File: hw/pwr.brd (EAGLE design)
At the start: 30.6 x 25.4 mm, 20 parts, among them IC1 MAX640, IC2 MAX640

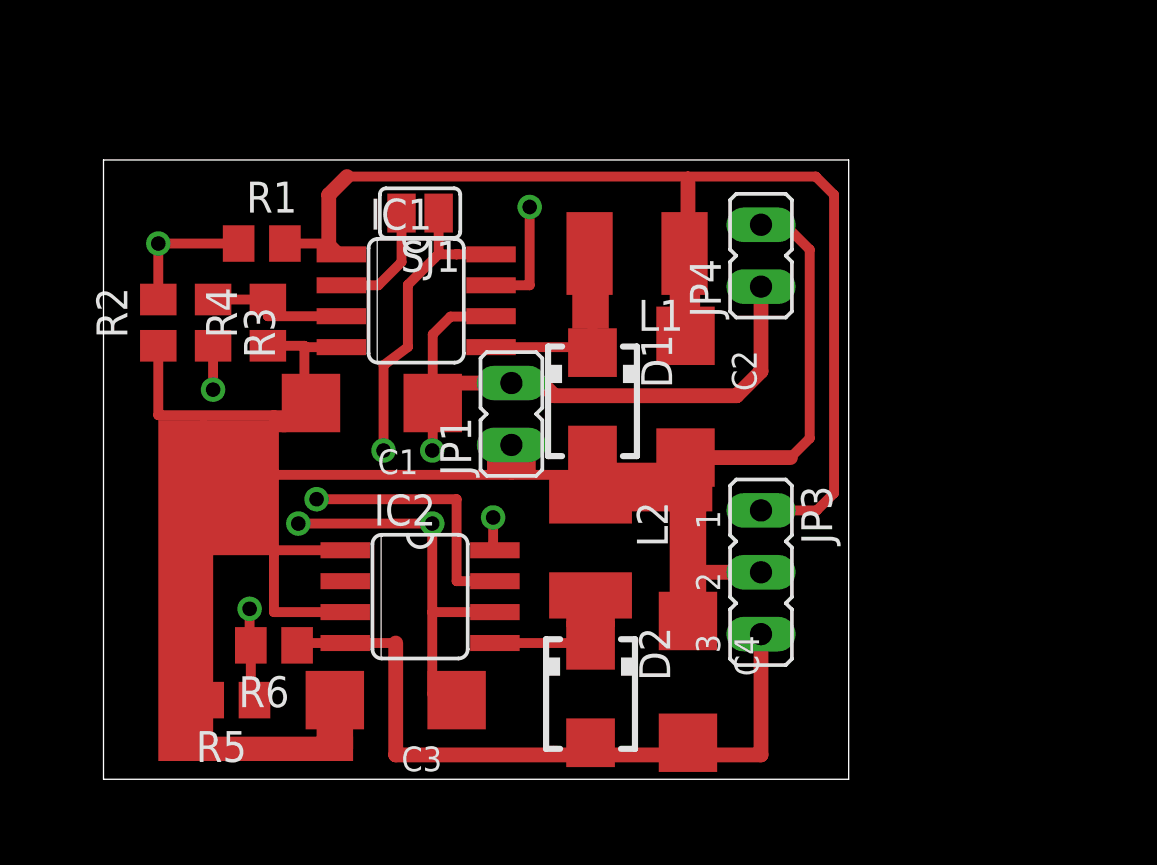
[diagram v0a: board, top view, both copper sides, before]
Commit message: Sargon rocks
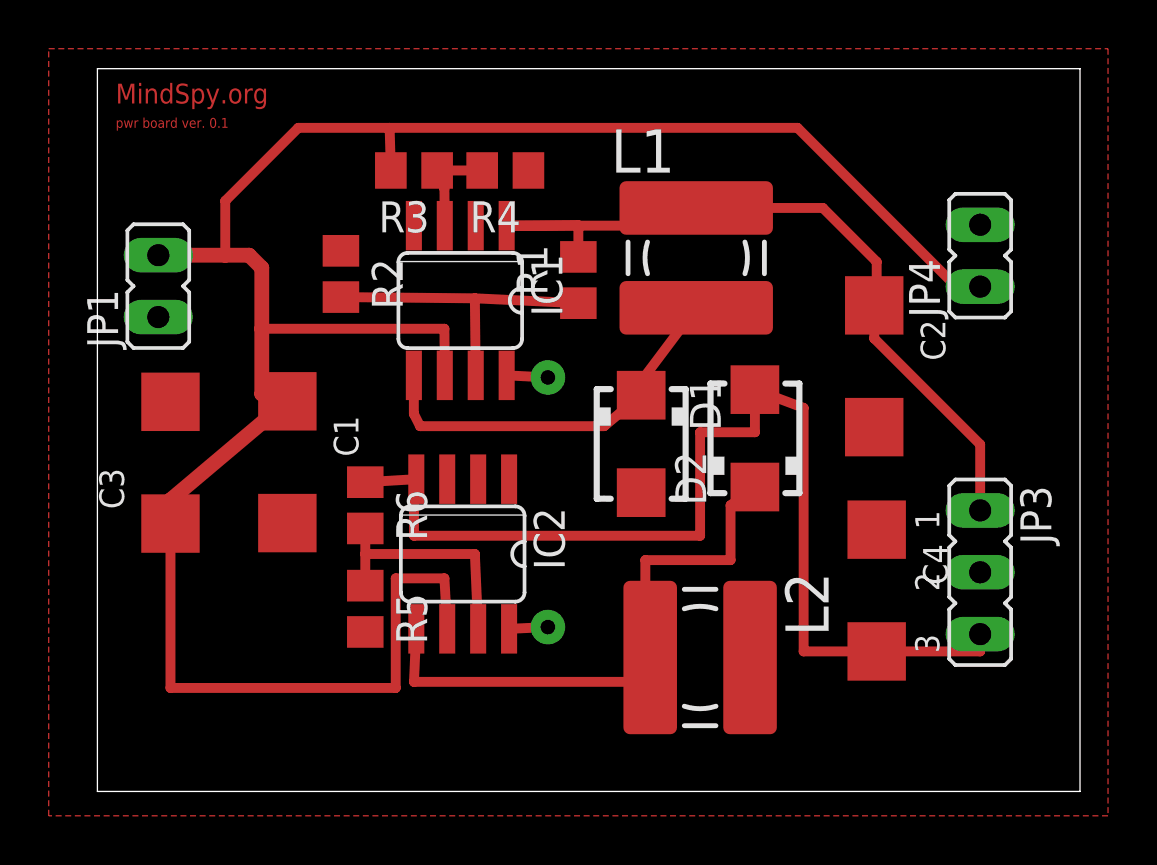
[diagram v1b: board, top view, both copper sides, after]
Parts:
- removed SJ1: (no value), jumper:SJ
- L1, L2: device rcl:L1812 -> rcl:POWER-CHOKE_WE-TPC
- moved JP1 15.4 mm to (2.25, 20.2)
- moved C3 13.4 mm to (2.75, 13.0), turned to 90 degrees
- moved R1 13.1 mm to (19.5, 20.5), turned to 90 degrees
- moved D2 12.5 mm to (26.8, 14.0), turned to 90 degrees
- moved R4 11.6 mm to (16.5, 25.0), turned to 180 degrees
- moved R3 10.4 mm to (12.8, 25.0), turned to 180 degrees
- moved JP3 9.00 mm to (36.0, 8.50)
- moved JP4 9.00 mm to (36.0, 21.5)
- moved C4 8.61 mm to (31.8, 7.75)
- moved C2 7.85 mm to (31.6, 17.0)
- moved R2 7.76 mm to (9.75, 20.8), turned to 270 degrees
- moved R6 6.86 mm to (10.8, 11.2), turned to 270 degrees
- moved R5 6.66 mm to (10.8, 7.00), turned to 270 degrees
- moved L2 6.36 mm to (24.5, 5.00)
- moved C1 4.24 mm to (7.55, 13.0), turned to 270 degrees
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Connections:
- removed net LBO: IC1.2, SJ1.2
- net SHDN: no longer SJ1.1
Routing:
- net GND: track 93.7 -> 0.00 mm
- net VBAT: track 43.8 -> 90.9 mm, vias 4 -> 0
- net N$4: track 5.98 -> 24.5 mm
- net +2V5: track 48.1 -> 32.7 mm
- net -2V5: track 29.7 -> 44.6 mm
- net SHDN: track 14.3 -> 3.29 mm
- net N$1: track 9.02 -> 16.0 mm
- net LBO: track 4.88 -> 0.00 mm
- net N$10: track 14.5 -> 10.1 mm, vias 2 -> 0
- net N$8: track 10.4 -> 13.2 mm, vias 2 -> 0
- net N$6: track 5.95 -> 4.17 mm
- added copper zone on layer 1, net GND
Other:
- board size 30.6 x 25.4 mm -> 40.4 x 29.7 mm
- board text removed: "+2V5"
- board text removed: "-2V5"
- board text removed: "AGND"
- board text removed: "DGND"
- board text removed: "LBO"
- board text removed: "SHDN"
- board text removed: "VBAT"
